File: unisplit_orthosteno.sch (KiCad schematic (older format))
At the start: 57 parts, among them U1 ProMicro

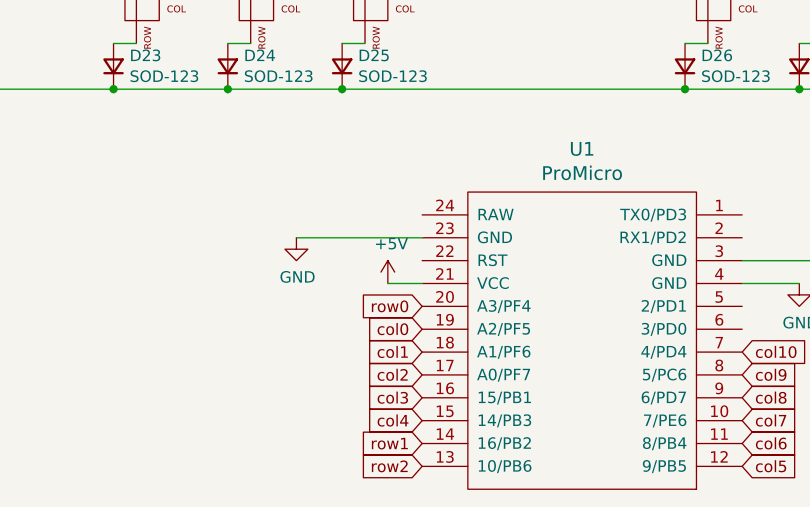
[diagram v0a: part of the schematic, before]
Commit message: finalize gerbers and create bom and place files for jlcpcb
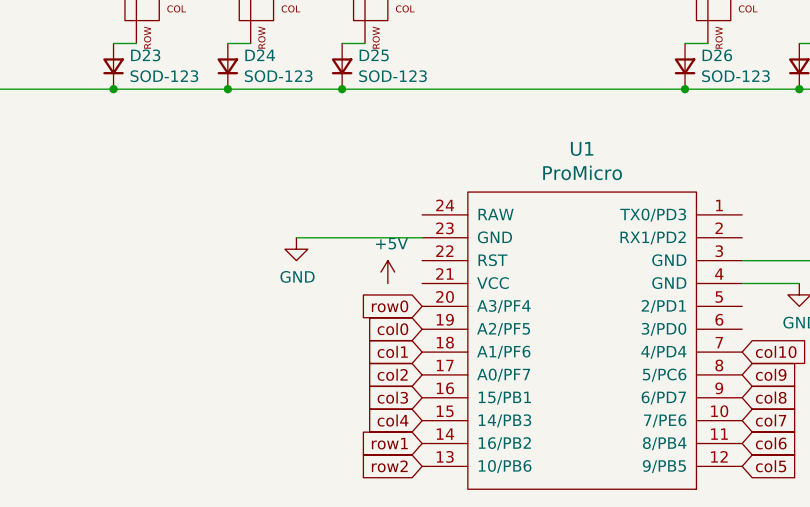
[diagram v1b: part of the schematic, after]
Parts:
- D1, D10, D11, D12, D13, D15, D16, D17, D18, D19, D2, D20, D21, D22, D23, D24, D25, D26, D27, D28, D3, D4, D5, D6, D7, D8, D9: LCSC (none) -> C81598
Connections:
- net +5V: no longer U1.21 (VCC)
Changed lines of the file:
@@
-$EndComp
-$Comp
-L Device:D_Small D1
-U 1 1 600ACFDD
-P 2450 2350
-F 0 "D1" V 2496 2280 50  0000 R CNN
-F 1 "SOD-123" V 2405 2280 50  0000 R CNN
-F 2 "Keebio-Parts:D_SOD123" V 2450 2350 50  0001 C CNN
-F 3 "~" V 2450 2350 50  0001 C CNN
-	1    2450 2350
-	0    -1   -1   0
 $EndComp
 $Comp
@@
 F 2 "Keebio-Parts:D_SOD123" V 2450 2850 50  0001 C CNN
 F 3 "~" V 2450 2850 50  0001 C CNN
+F 4 "C81598" V 2450 2850 50  0001 C CNN "LCSC"
 	1    2450 2850
 	0    -1   -1   0
@@
 F 2 "Keebio-Parts:D_SOD123" V 2950 2350 50  0001 C CNN
 F 3 "~" V 2950 2350 50  0001 C CNN
+F 4 "C81598" V 2950 2350 50  0001 C CNN "LCSC"
 	1    2950 2350
 	0    -1   -1   0
@@
 F 2 "Keebio-Parts:D_SOD123" V 2950 2850 50  0001 C CNN
 F 3 "~" V 2950 2850 50  0001 C CNN
+F 4 "C81598" V 2950 2850 50  0001 C CNN "LCSC"
 	1    2950 2850
 	0    -1   -1   0
@@
 F 2 "Keebio-Parts:D_SOD123" V 3450 2350 50  0001 C CNN
 F 3 "~" V 3450 2350 50  0001 C CNN
+F 4 "C81598" V 3450 2350 50  0001 C CNN "LCSC"
 	1    3450 2350
 	0    -1   -1   0
@@
 F 2 "Keebio-Parts:D_SOD123" V 3950 2350 50  0001 C CNN
 F 3 "~" V 3950 2350 50  0001 C CNN
+F 4 "C81598" V 3950 2350 50  0001 C CNN "LCSC"
 	1    3950 2350
 	0    -1   -1   0
@@
 F 2 "Keebio-Parts:D_SOD123" V 3950 2850 50  0001 C CNN
 F 3 "~" V 3950 2850 50  0001 C CNN
+F 4 "C81598" V 3950 2850 50  0001 C CNN "LCSC"
 	1    3950 2850
 	0    -1   -1   0
@@
 F 2 "Keebio-Parts:D_SOD123" V 4450 2350 50  0001 C CNN
 F 3 "~" V 4450 2350 50  0001 C CNN
+F 4 "C81598" V 4450 2350 50  0001 C CNN "LCSC"
 	1    4450 2350
 	0    -1   -1   0
@@
 F 2 "Keebio-Parts:D_SOD123" V 4450 2850 50  0001 C CNN
 F 3 "~" V 4450 2850 50  0001 C CNN
+F 4 "C81598" V 4450 2850 50  0001 C CNN "LCSC"
 	1    4450 2850
 	0    -1   -1   0
@@
 F 2 "Keebio-Parts:D_SOD123" V 5950 2350 50  0001 C CNN
 F 3 "~" V 5950 2350 50  0001 C CNN
+F 4 "C81598" V 5950 2350 50  0001 C CNN "LCSC"
 	1    5950 2350
 	0    -1   -1   0
@@
 F 2 "Keebio-Parts:D_SOD123" V 5950 2850 50  0001 C CNN
 F 3 "~" V 5950 2850 50  0001 C CNN
+F 4 "C81598" V 5950 2850 50  0001 C CNN "LCSC"
 	1    5950 2850
 	0    -1   -1   0
@@
 F 2 "Keebio-Parts:D_SOD123" V 6450 2350 50  0001 C CNN
 F 3 "~" V 6450 2350 50  0001 C CNN
+F 4 "C81598" V 6450 2350 50  0001 C CNN "LCSC"
 	1    6450 2350
 	0    -1   -1   0
@@
 F 2 "Keebio-Parts:D_SOD123" V 6450 2850 50  0001 C CNN
 F 3 "~" V 6450 2850 50  0001 C CNN
+F 4 "C81598" V 6450 2850 50  0001 C CNN "LCSC"
 	1    6450 2850
 	0    -1   -1   0
@@
 F 2 "Keebio-Parts:D_SOD123" V 6950 2350 50  0001 C CNN
 F 3 "~" V 6950 2350 50  0001 C CNN
+F 4 "C81598" V 6950 2350 50  0001 C CNN "LCSC"
 	1    6950 2350
 	0    -1   -1   0
@@
 F 2 "Keebio-Parts:D_SOD123" V 6950 2850 50  0001 C CNN
 F 3 "~" V 6950 2850 50  0001 C CNN
+F 4 "C81598" V 6950 2850 50  0001 C CNN "LCSC"
 	1    6950 2850
 	0    -1   -1   0
@@
 F 2 "Keebio-Parts:D_SOD123" V 7450 2350 50  0001 C CNN
 F 3 "~" V 7450 2350 50  0001 C CNN
+F 4 "C81598" V 7450 2350 50  0001 C CNN "LCSC"
 	1    7450 2350
 	0    -1   -1   0
@@
 F 2 "Keebio-Parts:D_SOD123" V 7450 2850 50  0001 C CNN
 F 3 "~" V 7450 2850 50  0001 C CNN
+F 4 "C81598" V 7450 2850 50  0001 C CNN "LCSC"
 	1    7450 2850
 	0    -1   -1   0
@@
 F 2 "Keebio-Parts:D_SOD123" V 7950 2350 50  0001 C CNN
 F 3 "~" V 7950 2350 50  0001 C CNN
+F 4 "C81598" V 7950 2350 50  0001 C CNN "LCSC"
 	1    7950 2350
 	0    -1   -1   0
@@
 F 2 "Keebio-Parts:D_SOD123" V 7950 2850 50  0001 C CNN
 F 3 "~" V 7950 2850 50  0001 C CNN
+F 4 "C81598" V 7950 2850 50  0001 C CNN "LCSC"
 	1    7950 2850
 	0    -1   -1   0
@@
 F 2 "Keebio-Parts:D_SOD123" V 8450 2350 50  0001 C CNN
 F 3 "~" V 8450 2350 50  0001 C CNN
+F 4 "C81598" V 8450 2350 50  0001 C CNN "LCSC"
 	1    8450 2350
 	0    -1   -1   0
@@
 F 2 "Keebio-Parts:D_SOD123" V 8450 2850 50  0001 C CNN
 F 3 "~" V 8450 2850 50  0001 C CNN
+F 4 "C81598" V 8450 2850 50  0001 C CNN "LCSC"
 	1    8450 2850
 	0    -1   -1   0
@@
 F 2 "Keebio-Parts:D_SOD123" V 3450 3600 50  0001 C CNN
 F 3 "~" V 3450 3600 50  0001 C CNN
+F 4 "C81598" V 3450 3600 50  0001 C CNN "LCSC"
 	1    3450 3600
 	0    -1   -1   0
@@
 F 2 "Keebio-Parts:D_SOD123" V 3950 3600 50  0001 C CNN
 F 3 "~" V 3950 3600 50  0001 C CNN
+F 4 "C81598" V 3950 3600 50  0001 C CNN "LCSC"
 	1    3950 3600
 	0    -1   -1   0
@@
 F 2 "Keebio-Parts:D_SOD123" V 5950 3600 50  0001 C CNN
 F 3 "~" V 5950 3600 50  0001 C CNN
+F 4 "C81598" V 5950 3600 50  0001 C CNN "LCSC"
 	1    5950 3600
 	0    -1   -1   0
@@
 F 2 "Keebio-Parts:D_SOD123" V 6450 3600 50  0001 C CNN
 F 3 "~" V 6450 3600 50  0001 C CNN
+F 4 "C81598" V 6450 3600 50  0001 C CNN "LCSC"
 	1    6450 3600
 	0    -1   -1   0
@@
 F 2 "Keebio-Parts:D_SOD123" V 4450 3600 50  0001 C CNN
 F 3 "~" V 4450 3600 50  0001 C CNN
+F 4 "C81598" V 4450 3600 50  0001 C CNN "LCSC"
 	1    4450 3600
 	0    -1   -1   0
@@
 F 2 "Keebio-Parts:D_SOD123" V 6950 3600 50  0001 C CNN
 F 3 "~" V 6950 3600 50  0001 C CNN
+F 4 "C81598" V 6950 3600 50  0001 C CNN "LCSC"
 	1    6950 3600
 	0    -1   -1   0
@@
 	4450 3700 5950 3700
 $Comp
-L power:GND #PWR?
+L power:GND #PWR0101
 U 1 1 601031E0
 P 4250 4350
-F 0 "#PWR?" H 4250 4100 50  0001 C CNN
+F 0 "#PWR0101" H 4250 4100 50  0001 C CNN
 F 1 "GND" H 4255 4177 50  0000 C CNN
 F 2 "" H 4250 4350 50  0001 C CNN
@@
 $EndComp
 $Comp
-L power:GND #PWR?
+L power:GND #PWR0102
 U 1 1 60103715
 P 6600 4450
-F 0 "#PWR?" H 6600 4200 50  0001 C CNN
+F 0 "#PWR0102" H 6600 4200 50  0001 C CNN
 F 1 "GND" H 6605 4277 50  0000 C CNN
 F 2 "" H 6600 4450 50  0001 C CNN
@@
 $EndComp
 $Comp
-L power:GND #PWR?
+L power:GND #PWR0103
 U 1 1 60103AAE
 P 6450 4550
-F 0 "#PWR?" H 6450 4300 50  0001 C CNN
+F 0 "#PWR0103" H 6450 4300 50  0001 C CNN
 F 1 "GND" H 6455 4377 50  0000 C CNN
 F 2 "" H 6450 4550 50  0001 C CNN
@@
 	6450 4550 6200 4550
 $Comp
-L power:+5V #PWR?
+L power:+5V #PWR0104
 U 1 1 6010D314
 P 4650 4550
-F 0 "#PWR?" H 4650 4400 50  0001 C CNN
+F 0 "#PWR0104" H 4650 4400 50  0001 C CNN
 F 1 "+5V" H 4665 4723 50  0000 C CNN
 F 2 "" H 4650 4550 50  0001 C CNN
@@
 	1    0    0    -1
 $EndComp
-Wire Wire Line
-	4650 4550 4800 4550
+$Comp
+L Device:D_Small D1
+U 1 1 600ACFDD
+P 2450 2350
+F 0 "D1" V 2496 2280 50  0000 R CNN
+F 1 "SOD-123" V 2405 2280 50  0000 R CNN
+F 2 "Keebio-Parts:D_SOD123" V 2450 2350 50  0001 C CNN
+F 3 "~" V 2450 2350 50  0001 C CNN
+F 4 "C81598" V 2450 2350 50  0001 C CNN "LCSC"
+	1    2450 2350
+	0    -1   -1   0
+$EndComp
 $EndSCHEMATC
